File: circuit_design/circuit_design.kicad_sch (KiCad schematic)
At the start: 1 part

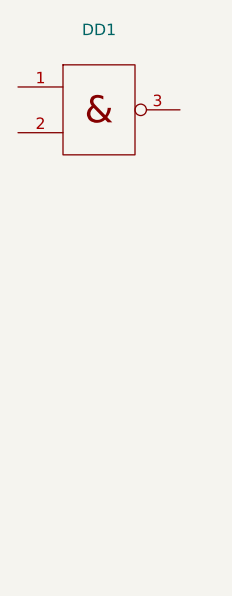
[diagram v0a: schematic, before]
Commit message: pr5
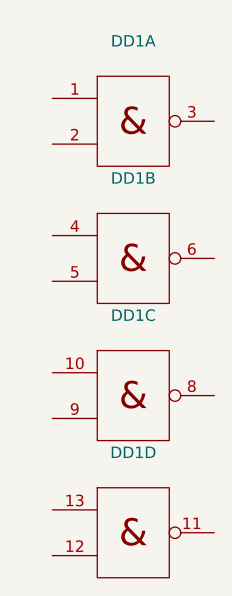
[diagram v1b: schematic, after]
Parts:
- added unit 3 of DD1
- added unit 2 of DD1
- added unit 4 of DD1
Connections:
- removed net Vcc: DD1.14 (Vcc)

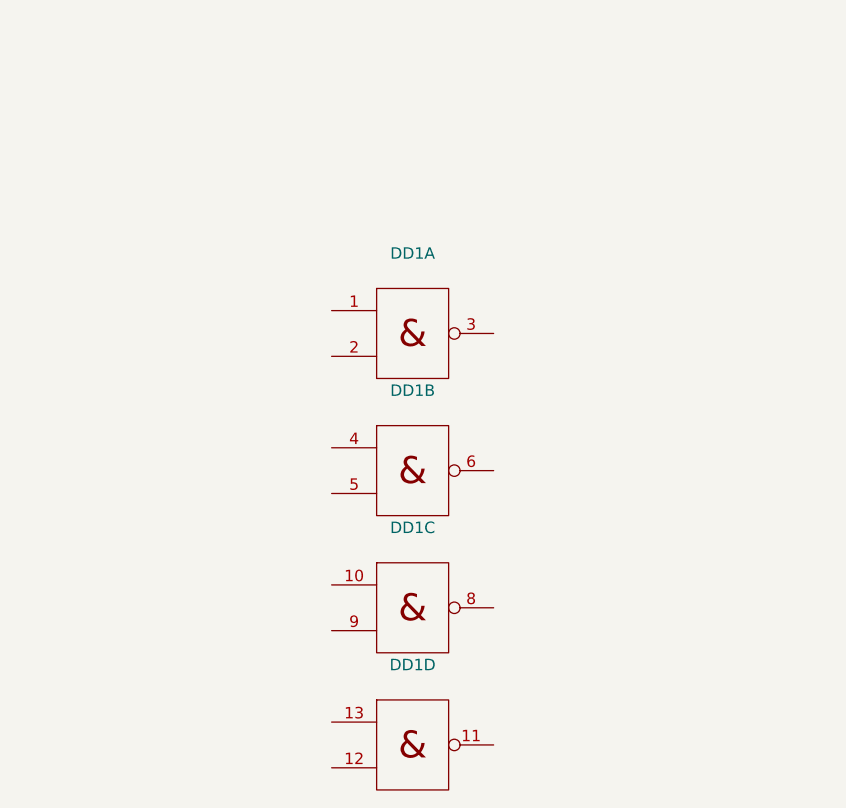
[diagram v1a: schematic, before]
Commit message: maybe 10?
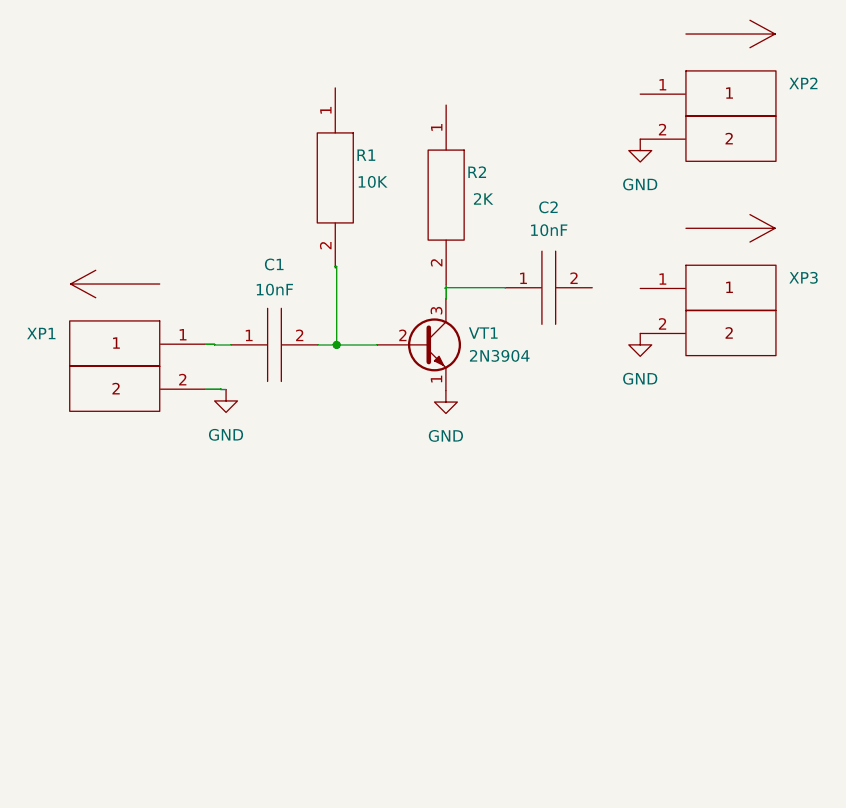
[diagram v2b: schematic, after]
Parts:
- removed DD1: ~, Pr4:К155ЛА3, symbol Pr4:К155ЛА3
- added C1, C2: 10nF, Pr2:CAP_CERAM_L5.0D0.8, symbol Pr2:Cap К10-17Б
- added R1: 10K, Pr2:RES_CONST_L6.0D0.8, symbol Pr2:Res MF 0.125
- added R2: 2K, Pr2:RES_CONST_L6.0D0.8, symbol Pr2:Res MF 0.125
- added VT1: 2N3904, Package_TO_SOT_THT:TO-92_Inline, symbol Transistor_BJT:2N3904
- added XP1, XP2, XP3: ~, Pr7:PLS-2, symbol pr7:PLS-2
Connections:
- new net: C1.2, VT1.2 (B)
- new net: C1.1, XP1.1
- new net GND: VT1.1 (E), XP2.2, XP3.2
